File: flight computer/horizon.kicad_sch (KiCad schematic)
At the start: 37 parts, among them J2 Conn_02x03_Counter_Clockwise, J7 Conn_02x03_Counter_Clockwise, J8 Conn_02x03_Counter_Clockwise, U1 MMCU, U3 NMCU, U4 TMCU, Y1 Crystal

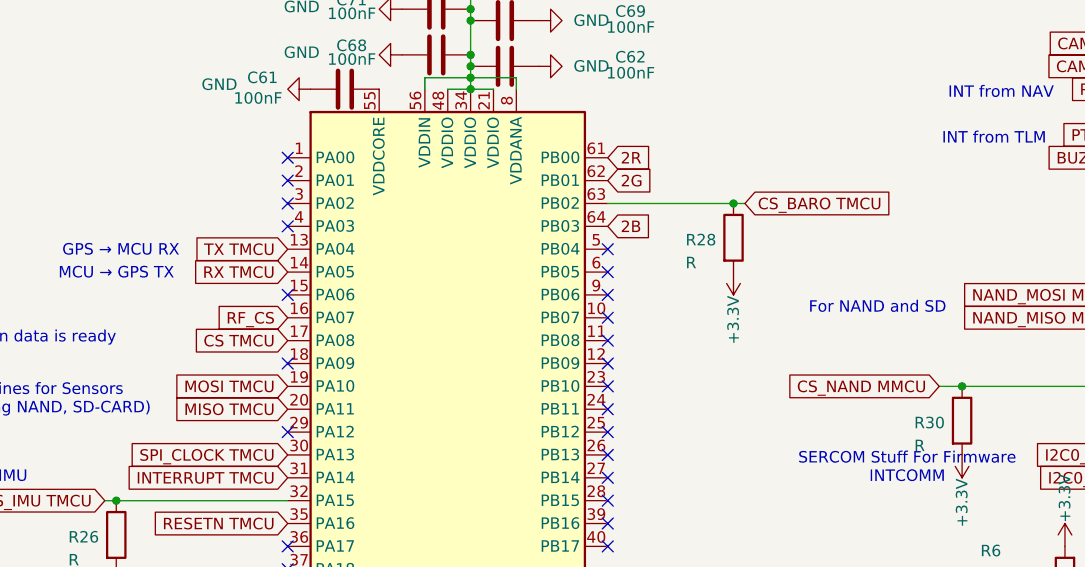
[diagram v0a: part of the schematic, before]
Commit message: Ummm, more baro routing to the MCU and stuff
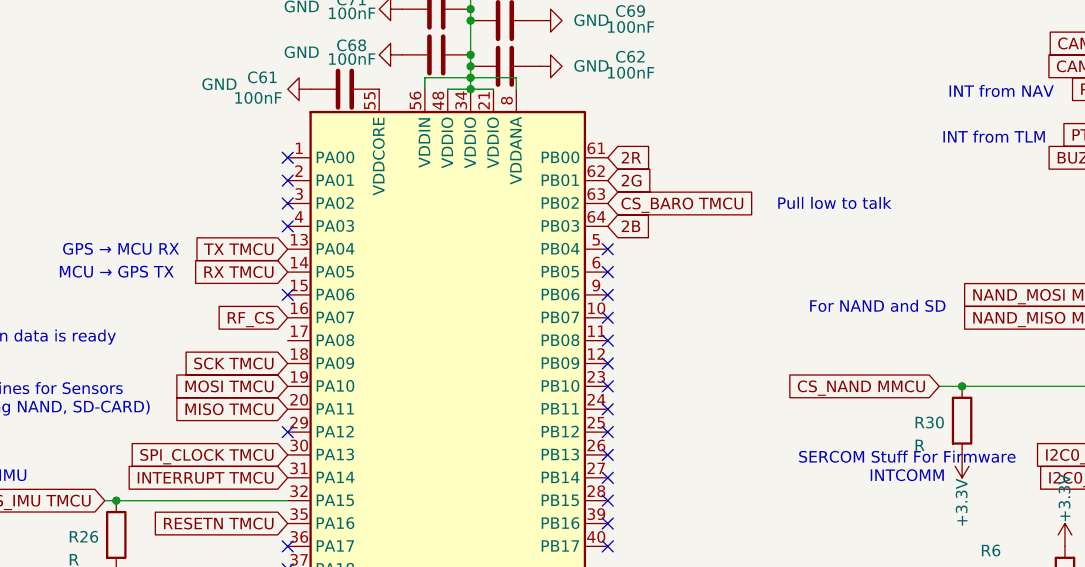
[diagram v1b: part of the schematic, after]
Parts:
- removed R28: R, Resistor_SMD:R_0603_1608Metric, symbol Device:R
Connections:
- net SCK TMCU: now reaches U4.18 (PA09)
- net CS TMCU: no longer names the net of U4.17 (PA08)
- no-connect marks 82 -> 81
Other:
- note added: "Pull low to talk"
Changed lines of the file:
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@@
 		)
 	)
+	(text "Pull low to talk"
+		(exclude_from_sim no)
+		(at 187.706 49.784 0)
+		(effects
+			(font
+				(size 1.27 1.27)
+			)
+		)
+	)
 	(text "GPS → MCU RX"
 		(exclude_from_sim no)
@@
 	)
 	(junction
-		(at 176.53 49.53)
-		(diameter 0)
-		(color 0 0 0 0)
-	)
-	(junction
 		(at 52.07 30.48)
 		(diameter 0)
@@
 	)
 	(no_connect
-		(at 127 67.31)
-	)
-	(no_connect
 		(at 31.75 86.36)
 	)
@@
 	(wire
 		(pts
-			(xy 176.53 49.53) (xy 162.56 49.53)
-		)
-		(stroke
-			(width 0)
-			(type default)
-		)
-	)
-	(wire
-		(pts
 			(xy 46.99 31.75) (xy 52.07 31.75)
 		)
@@
 	(wire
 		(pts
-			(xy 177.8 49.53) (xy 176.53 49.53)
-		)
-		(stroke
-			(width 0)
-			(type default)
-		)
-	)
-	(wire
-		(pts
 			(xy 147.32 35.56) (xy 147.32 36.83)
 		)
@@
 	(global_label "CS_BARO TMCU"
 		(shape input)
-		(at 177.8 49.53 0)
+		(at 162.56 49.53 0)
 		(fields_autoplaced yes)
 		(effects
@@
 		)
 		(property "Intersheetrefs" "${INTERSHEET_REFS}"
-			(at 195.1785 49.53 0)
+			(at 179.9385 49.53 0)
 			(effects
 				(font
@@
 		)
 	)
+	(global_label "SCK TMCU"
+		(shape input)
+		(at 127 67.31 180)
+		(fields_autoplaced yes)
+		(effects
+			(font
+				(size 1.27 1.27)
+			)
+			(justify right)
+		)
+		(property "Intersheetrefs" "${INTERSHEET_REFS}"
+			(at 114.2782 67.31 0)
+			(effects
+				(font
+					(size 1.27 1.27)
+				)
+				(justify right)
+				(hide yes)
+			)
+		)
+	)
 	(global_label "TX TMCU"
 		(shape input)
@@
 		)
 	)
-	(global_label "CS TMCU"
-		(shape input)
-		(at 127 64.77 180)
-		(fields_autoplaced yes)
-		(effects
-			(font
-				(size 1.27 1.27)
-			)
-			(justify right)
-		)
-		(property "Intersheetrefs" "${INTERSHEET_REFS}"
-			(at 115.5482 64.77 0)
-			(effects
-				(font
-					(size 1.27 1.27)
-				)
-				(justify right)
-				(hide yes)
-			)
-		)
-	)
 	(global_label "I2C0_SDA"
 		(shape input)
@@
 	)
 	(symbol
-		(lib_id "Device:R")
-		(at 176.53 53.34 0)
-		(unit 1)
-		(exclude_from_sim no)
-		(in_bom yes)
-		(on_board yes)
-		(dnp no)
-		(property "Reference" "R28"
-			(at 171.196 53.594 0)
-			(effects
-				(font
-					(size 1.27 1.27)
-				)
-				(justify left)
-			)
-		)
-		(property "Value" "R"
-			(at 171.196 56.134 0)
-			(effects
-				(font
-					(size 1.27 1.27)
-				)
-				(justify left)
-			)
-		)
-		(property "Footprint" "Resistor_SMD:R_0603_1608Metric"
-			(at 174.752 53.34 90)
-			(effects
-				(font
-					(size 1.27 1.27)
-				)
-				(hide yes)
-			)
-		)
-		(property "Datasheet" "~"
-			(at 176.53 53.34 0)
-			(effects
-				(font
-					(size 1.27 1.27)
-				)
-				(hide yes)
-			)
-		)
-		(property "Description" "Resistor"
-			(at 176.53 53.34 0)
-			(effects
-				(font
-					(size 1.27 1.27)
-				)
-				(hide yes)
-			)
-		)
-		(pin "2"
-		)
-		(pin "1"
-		)
-		(instances
-			(project "horizon"
-				(path "/78d9c2f3-deae-418a-8c21-4820ea8fc57f"
-					(reference "R28")
-					(unit 1)
-				)
-			)
-		)
-	)
-	(symbol
 		(lib_id "power:+3.3V")
 		(at 45.72 143.51 270)
@@
 					(unit 1)
 				)
-			)
-		)
-	)
-	(symbol
-		(lib_id "power:+3.3V")
-		(at 176.53 57.15 180)
-		(unit 1)
-		(exclude_from_sim no)
-		(in_bom yes)
-		(on_board yes)
-		(dnp no)
-		(property "Reference" "#PWR097"
-			(at 176.53 53.34 0)
-			(effects
-				(font
-					(size 1.27 1.27)
-				)
-				(hide yes)
-			)
-		)
-		(property "Value" "+3.3V"
-			(at 176.53 62.484 90)
-			(effects
-				(font
-					(size 1.27 1.27)
-				)
-			)
-		)
-		(property "Footprint" ""
-			(at 176.53 57.15 0)
-			(effects
-				(font
-					(size 1.27 1.27)
-				)
-				(hide yes)
-			)
-		)
-		(property "Datasheet" ""
-			(at 176.53 57.15 0)
-			(effects
-				(font
-					(size 1.27 1.27)
-				)
-				(hide yes)
-			)
-		)
-		(property "Description" "Power symbol creates a global label with name \"+3.3V\""
-			(at 176.53 57.15 0)
-			(effects
-				(font
-					(size 1.27 1.27)
-				)
-				(hide yes)
-			)
-		)
-		(pin "1"
-		)
-		(instances
-			(project "horizon"
-				(path "/78d9c2f3-deae-418a-8c21-4820ea8fc57f"
-					(reference "#PWR097")
-					(unit 1)
-				)

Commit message: wiring almost done
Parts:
- Y1: footprint Crystal:Crystal_SMD_0603-2Pin_6.0x3.5mm -> Crystal:Crystal_AT310_D3.0mm_L10.0mm_Vertical
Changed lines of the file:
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@@
 			)
 		)
-		(property "Footprint" "Crystal:Crystal_SMD_0603-2Pin_6.0x3.5mm"
+		(property "Footprint" "Crystal:Crystal_AT310_D3.0mm_L10.0mm_Vertical"
 			(at 279.4 91.44 0)
 			(effects

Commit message: for you scooter <3
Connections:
- net GND: now also J2.4 (Pin_4), J7.4 (Pin_4), J8.4 (Pin_4)
- net SWCLK DMCU-1: now also J7.6 (Pin_6); no longer J7.2 (Pin_2)
- net SWCLK DMCU-2: now also J8.6 (Pin_6); no longer J8.2 (Pin_2)
- net SWCLK MMCU: now also J2.6 (Pin_6); no longer J2.2 (Pin_2)
- net SWDIO DMCU-1: now also J7.2 (Pin_2); no longer J7.5 (Pin_5)
- net SWDIO DMCU-2: now also J8.2 (Pin_2); no longer J8.5 (Pin_5)
- net SWDIO MMCU: now also J2.2 (Pin_2); no longer J2.5 (Pin_5)
- net nRESET DMCU-1: now also J7.5 (Pin_5); no longer J7.4 (Pin_4)
- net nRESET DMCU-2: now also J8.5 (Pin_5); no longer J8.4 (Pin_4)
- net nRESET MMCU: now also J2.5 (Pin_5); no longer J2.4 (Pin_4)
- no-connect marks 81 -> 78
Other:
- moved on the sheet: C10, C17, C63, C64, C65, C66, C67, J2, J7, J8, R29, R3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

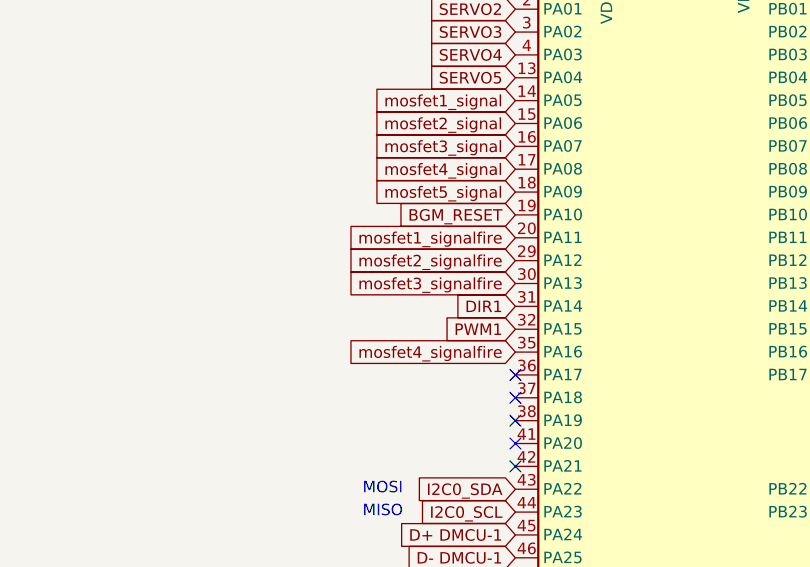
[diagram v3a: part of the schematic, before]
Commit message: idk, changes
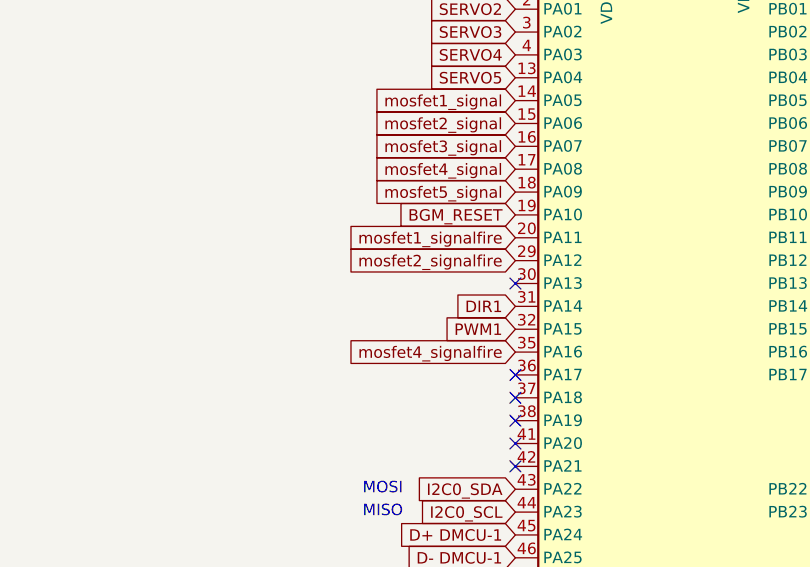
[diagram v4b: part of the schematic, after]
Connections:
- net mosfet3_signalfire: no longer names the net of U3.30 (PA13)
- no-connect marks 78 -> 79
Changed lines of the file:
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@@
+	)
+	(no_connect
+		(at 31.75 73.66)
 	)
 	(no_connect
@@
 			(effects
 				(font
-					(size 1.27 1.27)
-				)
-				(justify right)
-				(hide yes)
-			)
-		)
-	)
-	(global_label "mosfet3_signalfire"
-		(shape input)
-		(at 31.75 73.66 180)
-		(fields_autoplaced yes)
-		(effects
-			(font
-				(size 1.27 1.27)
-			)
-			(justify right)
-		)
-		(property "Intersheetrefs" "${INTERSHEET_REFS}"
-			(at 11.2269 73.66 0)
-			(effects
-				(font

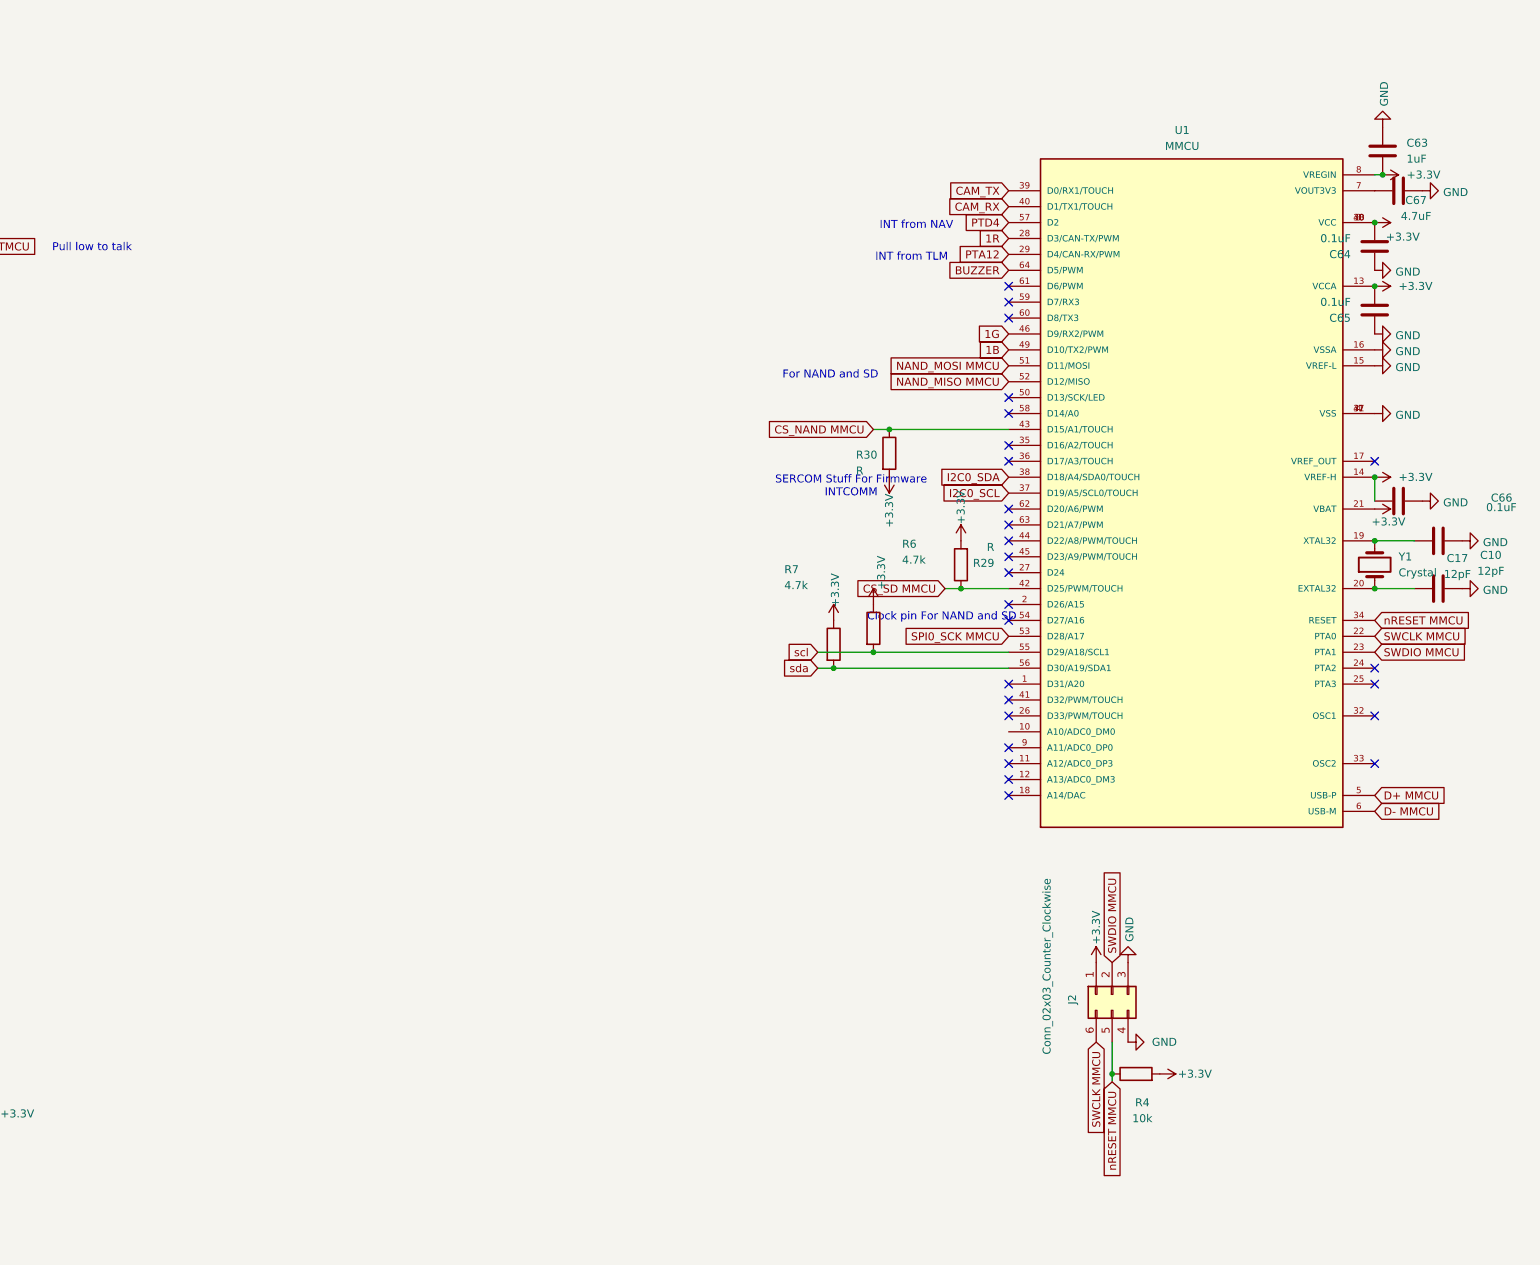
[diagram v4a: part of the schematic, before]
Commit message: drc
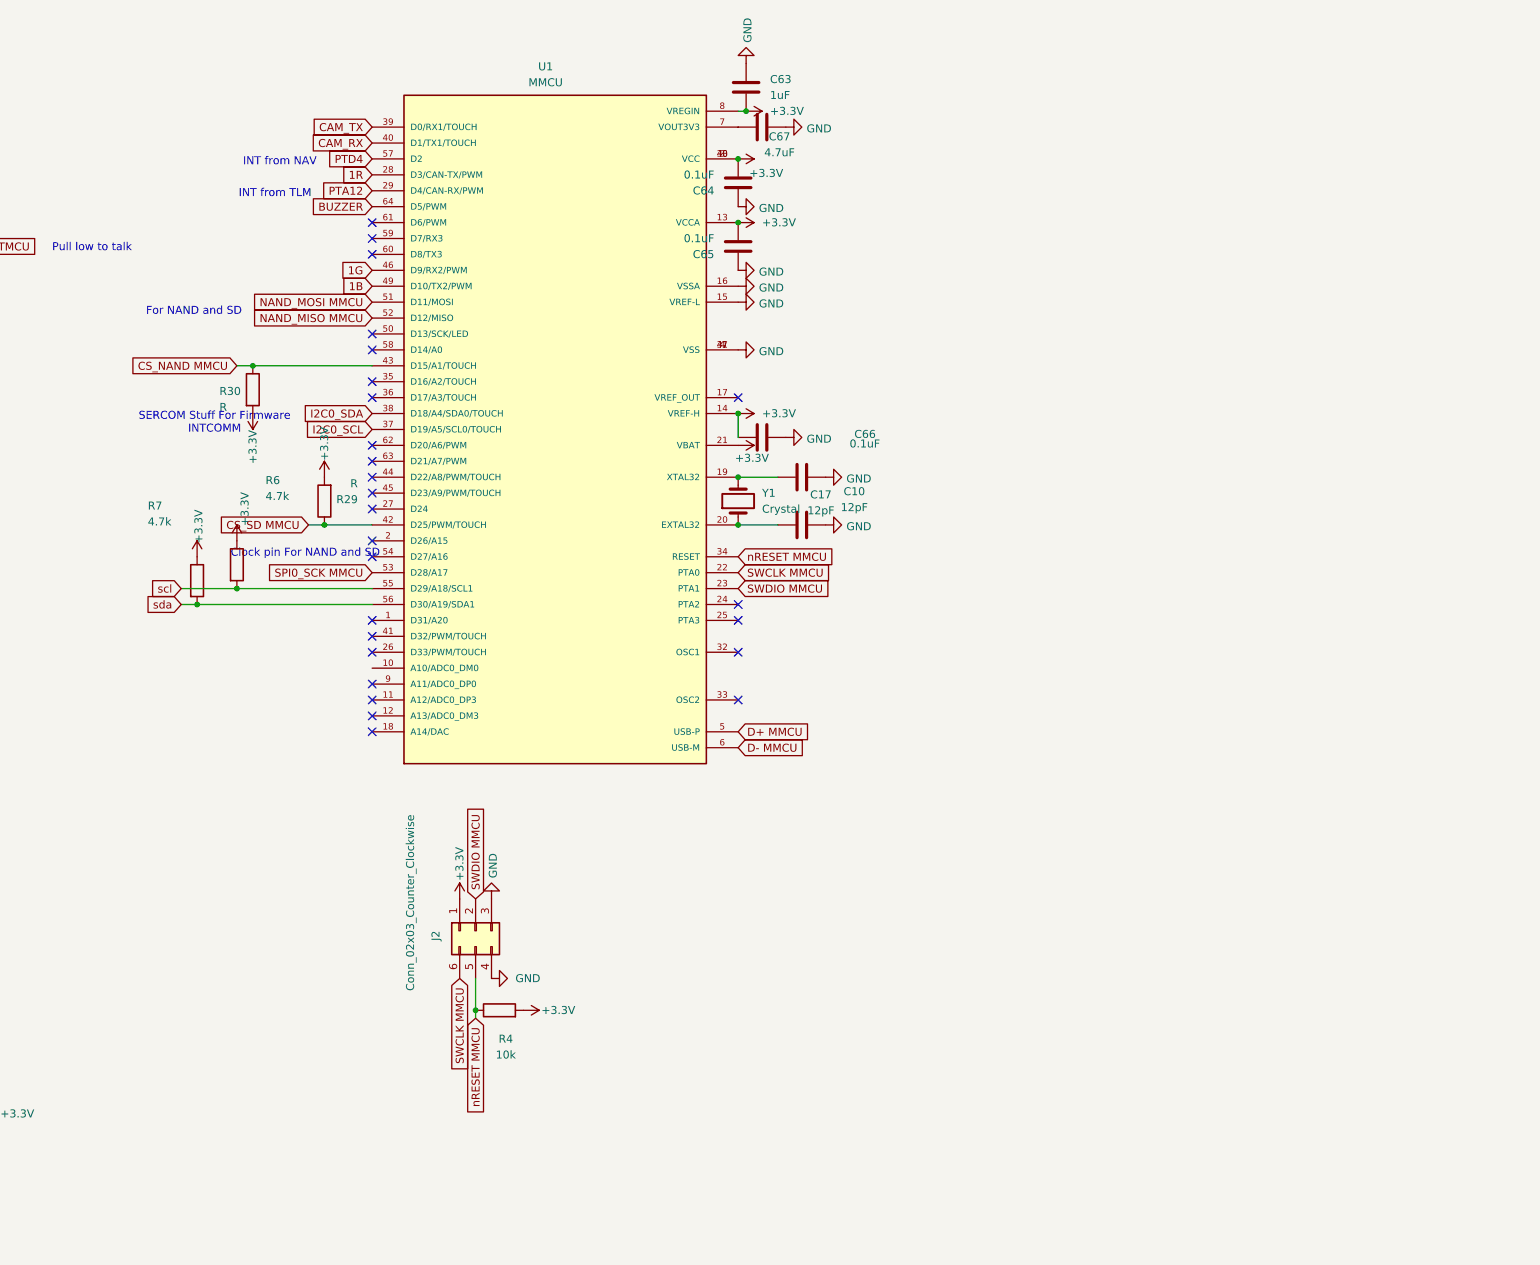
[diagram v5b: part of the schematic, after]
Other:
- moved on the sheet: C10, C17, C63, C64, C65, C66, C67, J2, R29, R30, R4, R6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
